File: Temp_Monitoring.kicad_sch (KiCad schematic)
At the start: 1 part

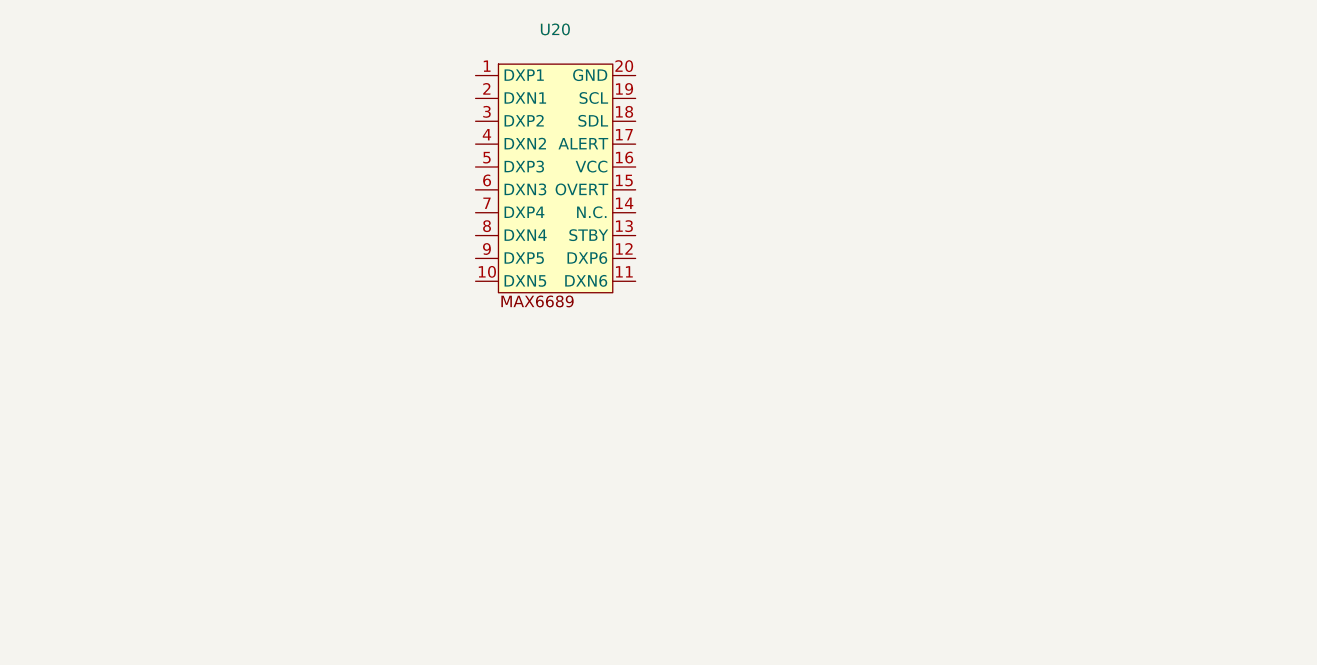
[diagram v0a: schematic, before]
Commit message: sch update done
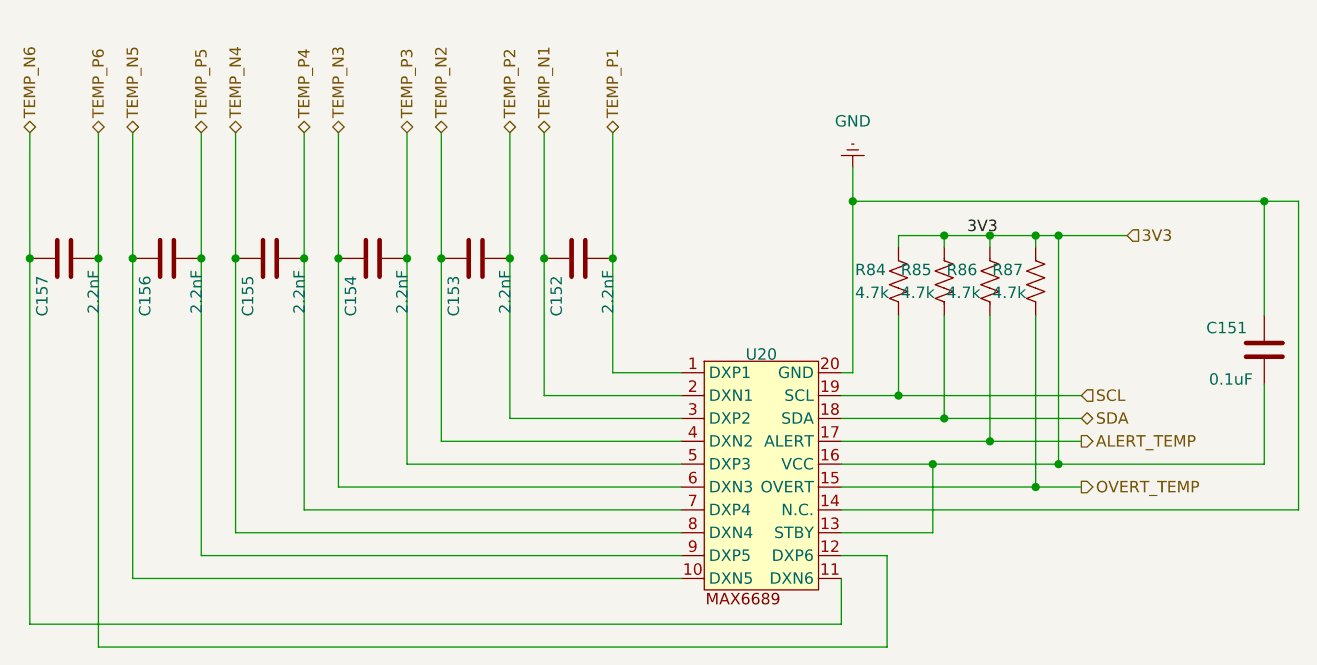
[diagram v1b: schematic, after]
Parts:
- added C151: 0.1uF, Capacitor_SMD:C_0402_1005Metric, symbol Device:C
- added C152, C153, C154, C155, C156, C157: 2.2nF, Capacitor_SMD:C_0402_1005Metric, symbol Device:C
- added R84, R85, R86, R87: 4.7k, Resistor_SMD:R_0402_1005Metric, symbol Device:R_US
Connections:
- net TEMP_P1: now reaches U20.1 (DXP1)
- net TEMP_P1: now also C152.1
- net TEMP_N5: now reaches U20.10 (DXN5)
- net TEMP_N5: now also C156.2
- net TEMP_N6: now reaches U20.11 (DXN6)
- net TEMP_N6: now also C157.2
- net TEMP_P6: now reaches U20.12 (DXP6)
- net TEMP_P6: now also C157.1
- net 3V3: now reaches U20.13 (STBY)
- net 3V3: now also U20.16 (VCC), C151.1, R84.2, R85.2, R86.2, R87.2
- net GND: now reaches U20.14 (N.C.)
- net GND: now also U20.20 (GND), C151.2
- net OVERT_TEMP: now reaches U20.15 (OVERT)
- net OVERT_TEMP: now also R87.1
- net ALERT_TEMP: now reaches U20.17 (ALERT)
- net ALERT_TEMP: now also R86.1
- net SDA: now reaches U20.18 (SDA)
- net SDA: now also R85.1
- net SCL: now reaches U20.19 (SCL)
- net SCL: now also R84.1
- net TEMP_N1: now reaches U20.2 (DXN1)
- net TEMP_N1: now also C152.2
- net TEMP_P2: now reaches U20.3 (DXP2)
- net TEMP_P2: now also C153.1
- net TEMP_N2: now reaches U20.4 (DXN2)
- net TEMP_N2: now also C153.2
- net TEMP_P3: now reaches U20.5 (DXP3)
- net TEMP_P3: now also C154.1
- net TEMP_N3: now reaches U20.6 (DXN3)
- net TEMP_N3: now also C154.2
- net TEMP_P4: now reaches U20.7 (DXP4)
- net TEMP_P4: now also C155.1
- net TEMP_N4: now reaches U20.8 (DXN4)
- net TEMP_N4: now also C155.2
- net TEMP_P5: now reaches U20.9 (DXP5)
- net TEMP_P5: now also C156.1

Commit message: Finish routing
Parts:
- U20: footprint (none) -> bitaxe:MAX6689UP9A+
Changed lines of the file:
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@@
 			)
 		)
-		(property "Footprint" ""
+		(property "Footprint" "bitaxe:MAX6689UP9A+"
 			(at 166.37 113.03 0)
 			(effects
@@
 			)
 		)
-		(property "Datasheet" ""
+		(property "Datasheet" "https://www.analog.com/media/en/technical-documentation/data-sheets/MAX6689.pdf"
 			(at 166.37 113.03 0)
 			(effects
